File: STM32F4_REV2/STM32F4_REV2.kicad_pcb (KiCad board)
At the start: 4 copper layers, 49.2 x 47.8 mm, 70 parts, among them IC1 MP2359DJ-LF-Z, J1 Screw_Terminal_01x02, J2 SWD, J3 Conn_01x04, J4 Conn_01x04, J5 USB_B_Micro, J6 Conn_01x04, J7 Conn_01x04, J8 Conn_01x02, Q1 AO3401A, SW1 SW_SPDT, SW2 SW_Push, U1 STM32F405RGT6, U2 USBLC6-2SC6, Y1 16MHz

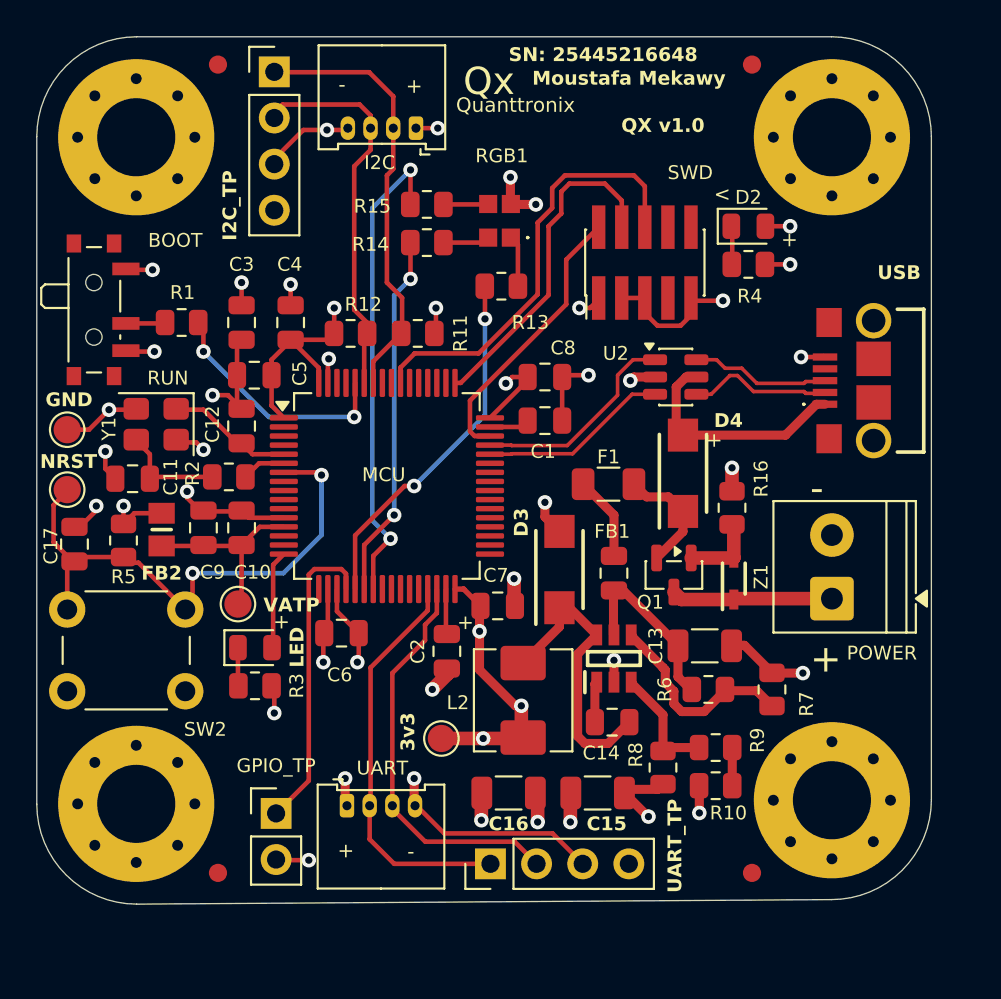
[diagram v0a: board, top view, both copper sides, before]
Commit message: Fixing most the bugs and following the checklist
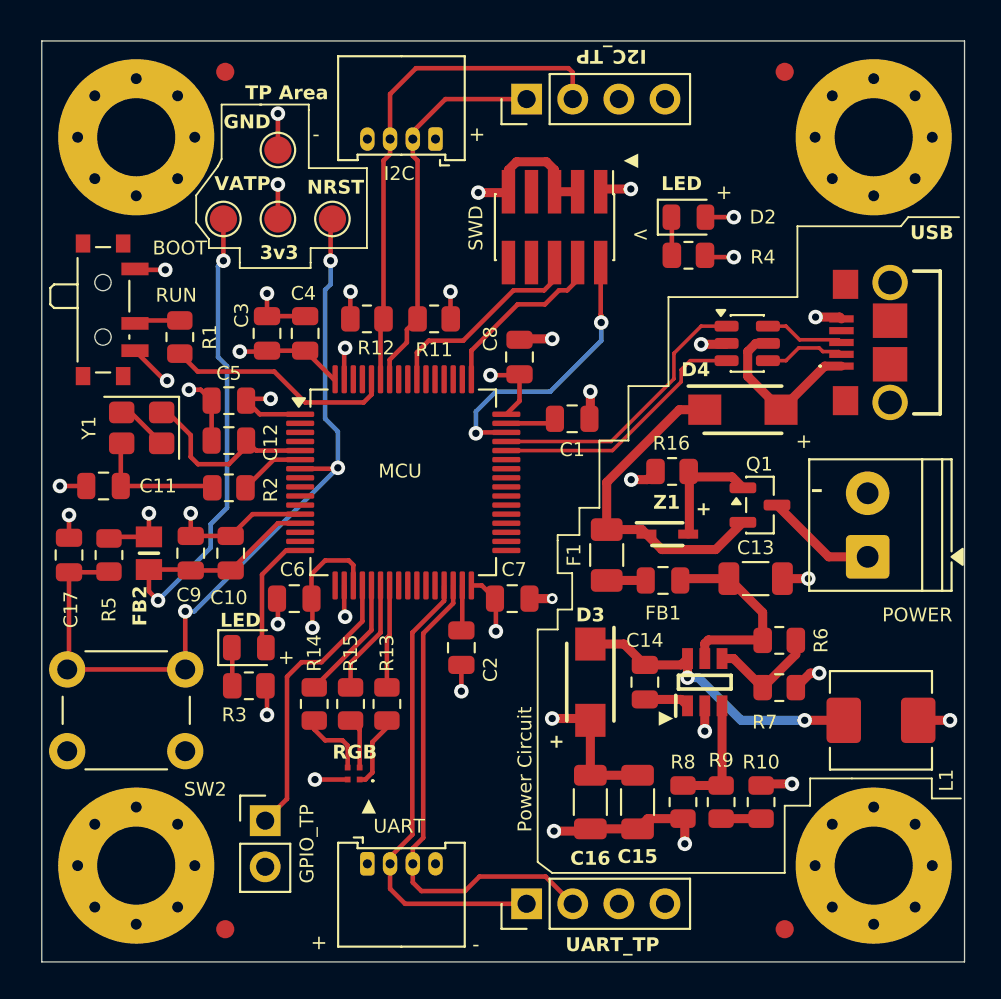
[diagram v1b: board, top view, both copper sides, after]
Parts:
- removed RGB1: 150080M153000, DownloadedLib:150080M153000
- added LED1: UHD111A-FKA-C3K23E1L3VG5ZB3Z3, M_Design_Lib:UHD111AFKAC3K23E1L3VG5ZB3Z3, F.Cu at (138.2, 114.5)
- D3, D4: footprint DownloadedLib:SODFL5226X110N -> M_Design_Lib:SODFL5226X110N
- FB1: value 600 @ 600 MHz -> 600 @ 100 MHz
- FB2: footprint DownloadedLib:BEADC2012X105N -> M_Design_Lib:BEADC2012X105N
- IC1: footprint DownloadedLib:MP2359DJ-LF-Z -> M_Design_Lib:MP2359DJ-LF-Z
- J5: footprint DownloadedLib:101181930001LF -> M_Design_Lib:101181930001LF
- R11, R12: value 4k7 -> 3k3
- R13, R15: value 1k -> 220
- R14: value 1k -> 330
- R7: value 68k -> 100k
- Z1: footprint DownloadedLib:SOD2512X110N -> M_Design_Lib:SOD2512X110N
- moved TP2 30.0 mm to (134.0, 84.0)
- moved R15 27.8 mm to (138.0, 110.7), turned to 90 degrees
- moved R14 26.1 mm to (136.0, 110.7), turned to 90 degrees
- moved R13 23.8 mm to (140.0, 110.7), turned to -90 degrees
- moved TP1 21.2 mm to (131.0, 84.0)
- moved TP4 20.9 mm to (137.0, 84.0)
- moved L1 19.7 mm to (167.2, 111.6), turned to 0 degrees
- moved TP3 19.3 mm to (134.0, 80.2)
- moved J7 14.0 mm to (147.7, 77.4), turned to 90 degrees
- moved D3 6.43 mm to (151.2, 109.5), turned to -90 degrees
- moved Q1 6.10 mm to (160.5, 99.8), turned to 0 degrees
- moved J2 5.34 mm to (149.2, 84.5), turned to -90 degrees
- moved IC1 5.17 mm to (157.5, 109.5)
- moved D4 4.81 mm to (159.6, 94.5), turned to 0 degrees
- moved R6 4.74 mm to (161.6, 107.2)
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- renumbered L2 to L1
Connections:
- R13 pad 1: Net-(RGB1-K_RED) -> RGB7_TP
- R13 pad 2: RGB5_TP -> Net-(LED1-CATHODE_BLUE)
- R14 pad 2: RGB6_TP -> RGB5_TP
- R15 pad 2: RGB7_TP -> RGB6_TP
- Z1 pad 1: +12V -> Net-(D4-K)
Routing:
- net +3.3VA: track 10.5 -> 34.2 mm, vias 0 -> 2
- net RGB7_TP: track 26.7 -> 5.67 mm, vias 2 -> 0
- net GND: track 81.3 -> 62.8 mm, vias 28 -> 25
- net NRST: track 30.9 -> 45.2 mm, vias 2 -> 3
- net RGB6_TP: track 20.1 -> 6.30 mm, vias 2 -> 0
- net RGB5_TP: track 20.0 -> 6.92 mm, vias 2 -> 0
- net SWO: track 24.1 -> 11.7 mm
- net Net-(D4-K): track 6.48 -> 18.2 mm
- net SWCLK: track 18.5 -> 9.99 mm
- net I2C1_SDA: track 21.5 -> 28.1 mm
- net +3.3V: track 57.3 -> 50.7 mm, vias 18 -> 16
- net Net-(IC1-EN): track 11.3 -> 6.26 mm
- net UART3_RX: track 22.3 -> 27.2 mm
- net USB_D-: track 10.5 -> 14.6 mm
- net Net-(LED1-CATHODE_BLUE): track 0.00 -> 4.05 mm
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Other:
- board size 49.2 x 47.8 mm -> 50.8 x 50.7 mm
- board text added: "Power Circuit"
- board text added: "RGB"
- board text added: "TP Area"
- board text added: "▲"
